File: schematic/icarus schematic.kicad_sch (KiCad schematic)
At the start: 54 parts, among them J1 Conn_01x02_Socket, J2 USB_C_Receptacle_USB2.0_16P, J3 Conn_01x02_Socket, J4 Conn_01x02_Socket, J5 Conn_01x02_Socket, Q1 AO3400A, Q2 AO3400A, Q3 AO3400A, Q4 AO3400A, SW1 SW_Push(BOOt), SW2 SW_Push(EN), U2 BMI088, U3 AMS1117-3.3, U4 ESP32-S3-WROOM-1

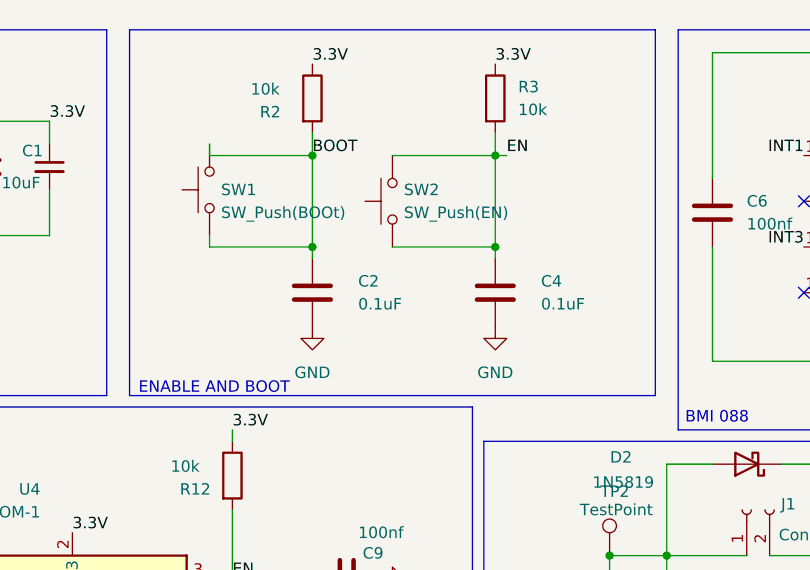
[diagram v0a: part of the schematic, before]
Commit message: kicad
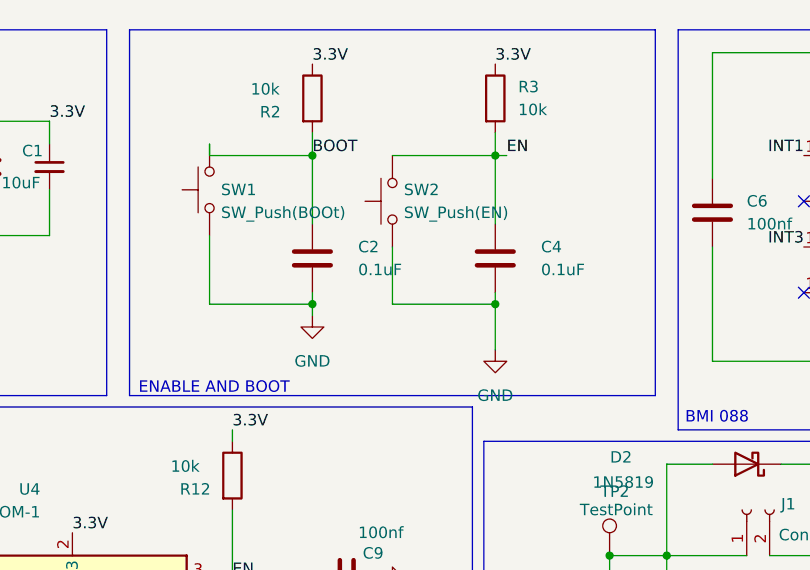
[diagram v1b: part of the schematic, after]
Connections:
- net BOOT: no longer SW1.1
- net EN: no longer SW2.1
- net GND: now also SW1.1, SW2.1
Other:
- moved on the sheet: C2, C4
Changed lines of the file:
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@@
 	)
 	(junction
-		(at 106.68 38.1)
-		(diameter 0)
-		(color 0 0 0 0)
-	)
-	(junction
 		(at 243.84 34.29)
 		(diameter 0)
@@
 	)
 	(junction
-		(at 86.36 27.94)
-		(diameter 0)
-		(color 0 0 0 0)
-	)
-	(junction
 		(at 143.51 135.89)
 		(diameter 0)
@@
 	)
 	(junction
+		(at 86.36 44.45)
+		(diameter 0)
+		(color 0 0 0 0)
+	)
+	(junction
 		(at 162.56 106.68)
 		(diameter 0)
@@
 	)
 	(junction
+		(at 86.36 27.94)
+		(diameter 0)
+		(color 0 0 0 0)
+	)
+	(junction
 		(at 279.4 21.59)
 		(diameter 0)
@@
 	)
 	(junction
+		(at 106.68 44.45)
+		(diameter 0)
+		(color 0 0 0 0)
+	)
+	(junction
 		(at 151.13 135.89)
 		(diameter 0)
@@
 	)
 	(junction
-		(at 86.36 38.1)
-		(diameter 0)
-		(color 0 0 0 0)
-	)
-	(junction
 		(at 162.56 72.39)
 		(diameter 0)
@@
 	(wire
 		(pts
+			(xy 86.36 43.18) (xy 86.36 44.45)
+		)
+		(stroke
+			(width 0)
+			(type default)
+		)
+	)
+	(wire
+		(pts
 			(xy 125.73 81.28) (xy 125.73 72.39)
 		)
@@
 	(wire
 		(pts
-			(xy 95.25 38.1) (xy 106.68 38.1)
-		)
-		(stroke
-			(width 0)
-			(type default)
-		)
-	)
-	(wire
-		(pts
 			(xy 40.64 102.87) (xy 44.45 102.87)
 		)
@@
 	(wire
 		(pts
-			(xy 106.68 27.94) (xy 106.68 38.1)
+			(xy 74.93 36.83) (xy 74.93 44.45)
 		)
 		(stroke
@@
 	(wire
 		(pts
+			(xy 95.25 38.1) (xy 95.25 44.45)
+		)
+		(stroke
+			(width 0)
+			(type default)
+		)
+	)
+	(wire
+		(pts
 			(xy 111.76 128.27) (xy 111.76 135.89)
 		)
@@
 	(wire
 		(pts
+			(xy 74.93 44.45) (xy 86.36 44.45)
+		)
+		(stroke
+			(width 0)
+			(type default)
+		)
+	)
+	(wire
+		(pts
 			(xy 173.99 81.28) (xy 170.18 81.28)
 		)
@@
 	(wire
 		(pts
-			(xy 86.36 38.1) (xy 86.36 39.37)
+			(xy 86.36 27.94) (xy 86.36 35.56)
 		)
 		(stroke
@@
 	(wire
 		(pts
+			(xy 86.36 45.72) (xy 86.36 44.45)
+		)
+		(stroke
+			(width 0)
+			(type default)
+		)
+	)
+	(wire
+		(pts
 			(xy 182.88 64.77) (xy 186.69 64.77)
 		)
@@
 	(wire
 		(pts
+			(xy 106.68 44.45) (xy 106.68 43.18)
+		)
+		(stroke
+			(width 0)
+			(type default)
+		)
+	)
+	(wire
+		(pts
 			(xy 256.54 59.69) (xy 256.54 62.23)
 		)
@@
 	(wire
 		(pts
-			(xy 86.36 27.94) (xy 86.36 38.1)
+			(xy 95.25 44.45) (xy 106.68 44.45)
 		)
 		(stroke
@@
 	(wire
 		(pts
-			(xy 74.93 38.1) (xy 74.93 36.83)
-		)
-		(stroke
-			(width 0)
-			(type default)
-		)
-	)
-	(wire
-		(pts
 			(xy 170.18 93.98) (xy 170.18 106.68)
 		)
@@
 	(wire
 		(pts
-			(xy 74.93 38.1) (xy 86.36 38.1)
+			(xy 180.34 106.68) (xy 187.96 106.68)
 		)
 		(stroke
@@
 	(wire
 		(pts
-			(xy 180.34 106.68) (xy 187.96 106.68)
+			(xy 151.13 16.51) (xy 151.13 20.32)
 		)
 		(stroke
@@
 	(wire
 		(pts
-			(xy 151.13 16.51) (xy 151.13 20.32)
+			(xy 186.69 72.39) (xy 186.69 81.28)
 		)
 		(stroke
@@
 	(wire
 		(pts
-			(xy 186.69 72.39) (xy 186.69 81.28)
+			(xy 106.68 101.6) (xy 106.68 139.7)
 		)
 		(stroke
@@
 	(wire
 		(pts
-			(xy 106.68 101.6) (xy 106.68 139.7)
+			(xy 243.84 39.37) (xy 243.84 41.91)
 		)
 		(stroke
@@
 	(wire
 		(pts
-			(xy 243.84 39.37) (xy 243.84 41.91)
+			(xy 151.13 16.51) (xy 130.81 16.51)
 		)
 		(stroke
@@
 	(wire
 		(pts
-			(xy 151.13 16.51) (xy 130.81 16.51)
+			(xy 106.68 49.53) (xy 106.68 44.45)
 		)
 		(stroke
@@
 	(wire
 		(pts
-			(xy 106.68 38.1) (xy 106.68 39.37)
+			(xy 106.68 27.94) (xy 106.68 35.56)
 		)
 		(stroke
@@
 	(symbol
 		(lib_id "Device:C")
-		(at 106.68 43.18 0)
+		(at 106.68 39.37 0)
 		(unit 1)
 		(body_style 1)
@@
 		(fields_autoplaced yes)
 		(property "Reference" "C4"
-			(at 111.76 41.9099 0)
+			(at 111.76 38.0999 0)
 			(show_name no)
 			(do_not_autoplace no)
@@
 		)
 		(property "Value" "0.1uF"
-			(at 111.76 44.4499 0)
+			(at 111.76 40.6399 0)
 			(show_name no)
 			(do_not_autoplace no)
@@
 		)
 		(property "Footprint" "Capacitor_SMD:C_0402_1005Metric_Pad0.74x0.62mm_HandSolder"
-			(at 107.6452 46.99 0)
+			(at 107.6452 43.18 0)
 			(hide yes)
 			(show_name no)
@@
 		)
 		(property "Datasheet" ""
-			(at 106.68 43.18 0)
+			(at 106.68 39.37 0)
 			(hide yes)
 			(show_name no)
@@
 		)
 		(property "Description" "Unpolarized capacitor"
-			(at 106.68 43.18 0)
+			(at 106.68 39.37 0)
 			(hide yes)
 			(show_name no)
@@
 	(symbol
 		(lib_id "power:GND")
-		(at 106.68 46.99 0)
+		(at 106.68 49.53 0)
 		(unit 1)
 		(body_style 1)
@@
 		(fields_autoplaced yes)
 		(property "Reference" "#PWR08"
-			(at 106.68 53.34 0)
+			(at 106.68 55.88 0)
 			(hide yes)
 			(show_name no)
@@
 		)
 		(property "Value" "GND"
-			(at 106.68 52.07 0)
+			(at 106.68 54.61 0)
 			(show_name no)
 			(do_not_autoplace no)
@@
 		)
 		(property "Footprint" ""
-			(at 106.68 46.99 0)
+			(at 106.68 49.53 0)
 			(hide yes)
 			(show_name no)
@@
 		)
 		(property "Datasheet" ""
-			(at 106.68 46.99 0)
+			(at 106.68 49.53 0)
 			(hide yes)
 			(show_name no)
@@
 		)
 		(property "Description" "Power symbol creates a global label with name \"GND\" , ground"
-			(at 106.68 46.99 0)
+			(at 106.68 49.53 0)
 			(hide yes)
 			(show_name no)
@@
 	(symbol
 		(lib_id "power:GND")
-		(at 86.36 46.99 0)
+		(at 86.36 45.72 0)
 		(unit 1)
 		(body_style 1)
@@
 		(fields_autoplaced yes)
 		(property "Reference" "#PWR07"
-			(at 86.36 53.34 0)
+			(at 86.36 52.07 0)
 			(hide yes)
 			(show_name no)
@@
 		)
 		(property "Value" "GND"
-			(at 86.36 52.07 0)
+			(at 86.36 50.8 0)
 			(show_name no)
 			(do_not_autoplace no)
@@
 		)
 		(property "Footprint" ""
-			(at 86.36 46.99 0)
+			(at 86.36 45.72 0)
 			(hide yes)
 			(show_name no)
@@
 		)
 		(property "Datasheet" ""
-			(at 86.36 46.99 0)
+			(at 86.36 45.72 0)
 			(hide yes)
 			(show_name no)
@@
 		)
 		(property "Description" "Power symbol creates a global label with name \"GND\" , ground"
-			(at 86.36 46.99 0)
+			(at 86.36 45.72 0)
 			(hide yes)
 			(show_name no)
@@
 	(symbol
 		(lib_id "Device:C")
-		(at 86.36 43.18 0)
+		(at 86.36 39.37 0)
 		(unit 1)
 		(body_style 1)
@@
 		(fields_autoplaced yes)
 		(property "Reference" "C2"
-			(at 91.44 41.9099 0)
+			(at 91.44 38.0999 0)
 			(show_name no)
 			(do_not_autoplace no)
@@
 		)
 		(property "Value" "0.1uF"
-			(at 91.44 44.4499 0)
+			(at 91.44 40.6399 0)
 			(show_name no)
 			(do_not_autoplace no)
@@
 		)
 		(property "Footprint" "Capacitor_SMD:C_0402_1005Metric_Pad0.74x0.62mm_HandSolder"
-			(at 87.3252 46.99 0)
+			(at 87.3252 43.18 0)
 			(hide yes)
 			(show_name no)
@@
 		)
 		(property "Datasheet" ""
-			(at 86.36 43.18 0)
+			(at 86.36 39.37 0)
 			(hide yes)
 			(show_name no)
@@
 		)
 		(property "Description" "Unpolarized capacitor"
-			(at 86.36 43.18 0)
+			(at 86.36 39.37 0)
 			(hide yes)
 			(show_name no)
